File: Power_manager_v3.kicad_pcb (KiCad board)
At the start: 4 copper layers, 50 x 25 mm, 94 parts, among them J1 L_input, J2 Pow_mng_pow, J3 Load1, J4 Load2, J5 SWD (PLS5), J6 Dig_mod_iface, Q1 2N5551S, Q2 2N5551S, Q3 BSS138, U1 DC12003, U2 G3MB-202PL, U3 G3MB-202PL, U4 STM32F030F4Px, U5 HLW8112, U6 ADuM1251ARZ, U7 ADuM1201AR, U8 LM1117-3.3, Y1 CSTCE8M, Y2 ABLS-3.579545MHZ-D-3-Y-T

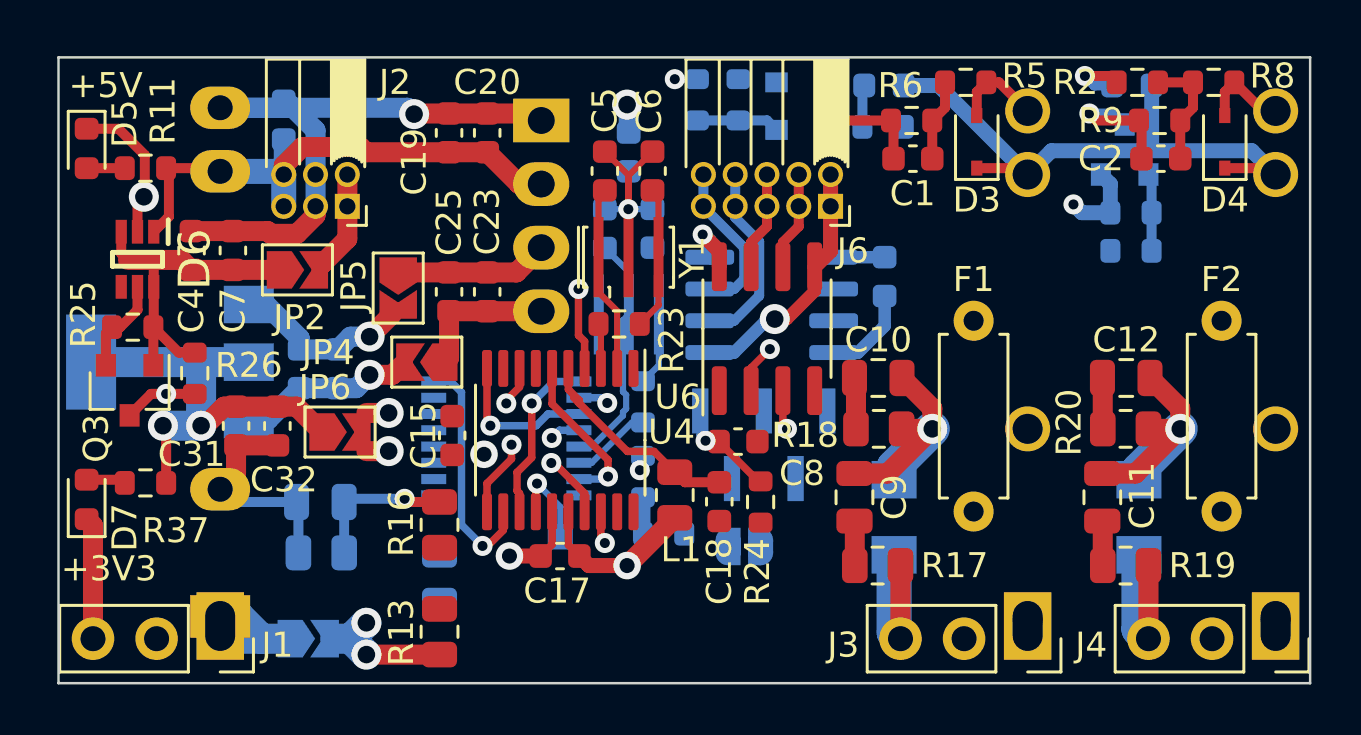
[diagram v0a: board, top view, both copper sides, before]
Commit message: Окончена трассировка печатной платы
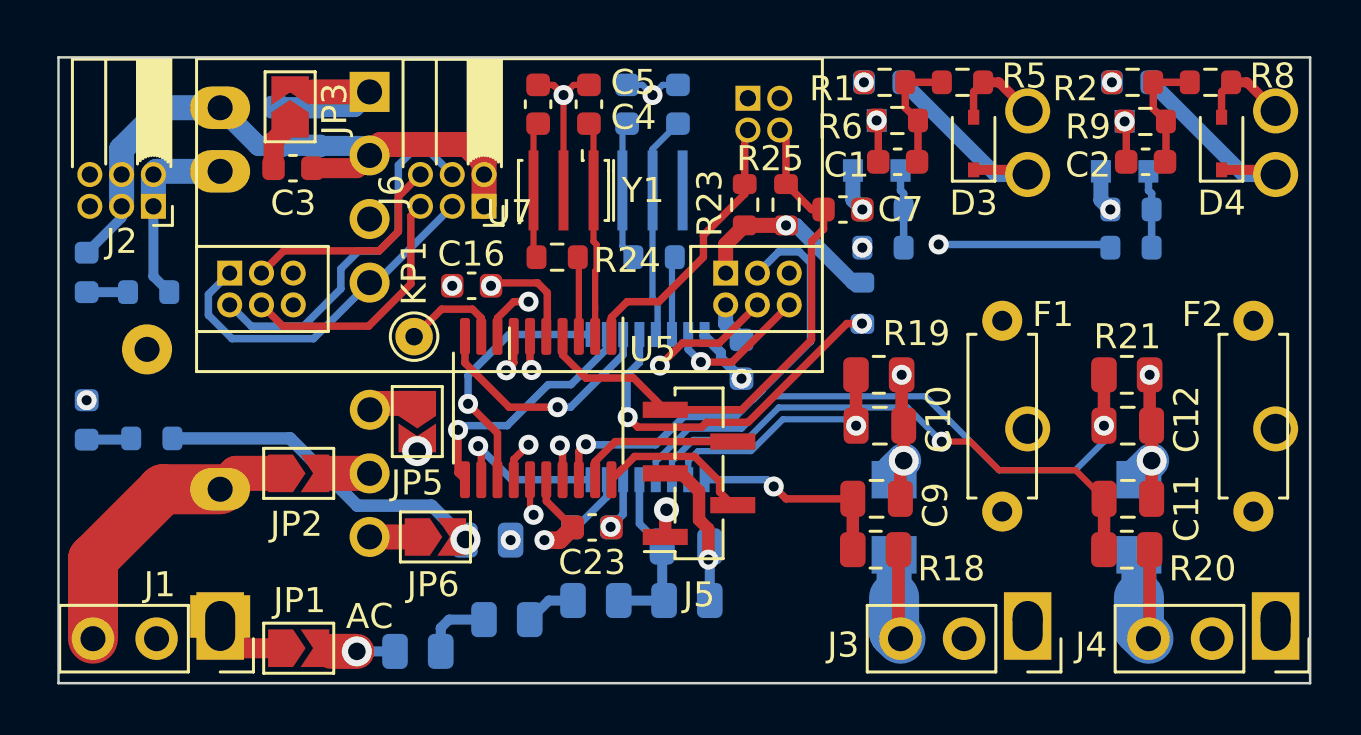
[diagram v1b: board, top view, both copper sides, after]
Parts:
- removed C19, C25, C27, C32: 10uF, Capacitor_SMD:C_0603_1608Metric
- removed C20, C24, C28, C30, C31: 100nF, Capacitor_SMD:C_0603_1608Metric
- removed C21, C22: 22pF, Capacitor_SMD:C_0603_1608Metric
- removed D7: +3.3V, LED_SMD:LED_0603_1608Metric
- removed PS1: B0505S, Modules:B0505S
- removed Q3: BSS138, Package_TO_SOT_SMD:SOT-23
- removed the R16 at (90.2, 93.7)
- removed the R21 at (85.5, 94.8)
- removed R28, R37: 10k, Resistor_SMD:R_0603_1608Metric
- removed U8: LM1117-3.3, Package_TO_SOT_SMD:SOT-223-3_TabPin2
- added C14: 100nF, Capacitor_SMD:C_0603_1608Metric, B.Cu at (96.3, 93.8)
- added C16: 100nF, Capacitor_SMD:C_0603_1608Metric, F.Cu at (91.5, 84.1)
- added GND1: TestPoint_Small, TestPoint:TestPoint_THTPad_D2.0mm_Drill1.0mm, B.Cu at (78.5, 86.7)
- added R14: 10k, Resistor_SMD:R_0603_1608Metric, B.Cu at (78.7, 90.2)
- added R17: 332k, Resistor_SMD:R_0805_2012Metric, B.Cu at (96.5, 96.7)
- C15, C8, L1: moved to B.Cu
- C17, C18: value 100nF -> 22pF; moved to B.Cu
- C3, J5, JP1, R1: moved to F.Cu
- C4: value 100nF -> 10pF
- C6: value 10pF -> 10uF; moved to B.Cu
- C7: value 10uF -> 100nF
- D5: value +5P -> +5V; moved to B.Cu
- D6: value LM66100DCKR -> +3.3VP; footprint Modules:SOP65P210X110-6N -> LED_SMD:LED_0603_1608Metric; moved to B.Cu
- J6: footprint Connector_PinSocket_1.27mm:PinSocket_2x05_P1.27mm_Horizontal -> Connector_PinSocket_1.27mm:PinSocket_2x03_P1.27mm_Horizontal
- JP2: value 5V_en -> N_en
- JP3: value BOOT0 -> 5V_en; footprint Jumper:SolderJumper-2_P1.3mm_Open_RoundedPad1.0x1.5mm -> Jumper:SolderJumper-2_P1.3mm_Open_TrianglePad1.0x1.5mm; moved to F.Cu
- JP4: value 5VL_en -> Jumper_2x2_Open; footprint Jumper:SolderJumper-2_P1.3mm_Open_TrianglePad1.0x1.5mm -> Modules:PinHeader_2x02_P1.27mm_Vertical; moved to B.Cu
- JP5: value N_en -> 5VP_en
- JP6: value 3V3_en -> 3.3VP_en
- KP1: footprint TestPoint:TestPoint_Pad_1.0x1.0mm -> TestPoint:TestPoint_THTPad_D1.5mm_Drill0.7mm; moved to F.Cu
- R11: value 10k -> 332k; footprint Resistor_SMD:R_0603_1608Metric -> Resistor_SMD:R_0805_2012Metric; moved to B.Cu
- R13: value 332k -> 10k; footprint Resistor_SMD:R_0805_2012Metric -> Resistor_SMD:R_0603_1608Metric; moved to B.Cu
- R22: value 10k -> 1k; footprint Resistor_SMD:R_0603_1608Metric -> Resistor_SMD:R_0805_2012Metric
- R23, R27: value 50 -> 10k
- R24: value 10k -> 50
- R26: value 2.2M -> 50; moved to B.Cu
- U4: value STM32F030F4Px -> DC5V_DC5V3V3_v3; footprint Package_SO:TSSOP-20_4.4x6.5mm_P0.65mm -> Modules:DC5V_DC5V3V3_v3; moved to B.Cu
- U5: value HLW8112 -> STM32F030F4Px; footprint Package_SO:SSOP-16_4.4x5.2mm_P0.65mm -> Package_SO:TSSOP-20_4.4x6.5mm_P0.65mm; moved to F.Cu
- U6: value ADuM1251ARZ -> HLW8112; footprint Package_SO:SOIC-8_3.9x4.9mm_P1.27mm -> Package_SO:SSOP-16_4.4x5.2mm_P0.65mm; moved to B.Cu
- U7: value ADuM1201AR -> ADuM_I2C_v3; footprint Package_SO:SOIC-8_3.9x4.9mm_P1.27mm -> Modules:ADuM_I2C_Horizontal; moved to F.Cu
- moved R25 26.6 mm to (104.1, 80.9), turned to 90 degrees
- moved JP3 25.3 mm to (84.3, 77.0), turned to 90 degrees
- moved C7 24.4 mm to (106.3, 81.1), turned to 0 degrees
- moved R11 23.1 mm to (92.9, 97.5), turned to 180 degrees
- moved C8 22.3 mm to (83.7, 77.8), turned to 90 degrees
- moved R26 18.9 mm to (98.8, 83.0), turned to 180 degrees
- moved C17 18.7 mm to (99.7, 76.9), turned to 270 degrees
- moved R13 17.9 mm to (78.6, 84.4), turned to 0 degrees
- moved C4 16.9 mm to (96.2, 76.9), turned to 90 degrees
- moved JP4 16.6 mm to (102.5, 76.6), turned to 270 degrees
- moved C18 16.3 mm to (97.7, 76.9), turned to 270 degrees
- moved C13 14.7 mm to (100.1, 94.5), turned to 180 degrees
- moved J6 13.8 mm to (92.0, 81.0)
- moved C6 13.6 mm to (85.3, 77.8)
- moved R24 12.7 mm to (94.9, 83.0), turned to 0 degrees
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- renumbered R14 to R15, R15 to R16, R17 to R18, R18 to R19, R19 to R20, R20 to R21
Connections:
- C15 pad 2: Net-(C15-Pad2) -> +3.3VP
- C17 pad 2: +3.3VP -> Net-(C17-Pad2)
- C23 pad 1: Net-(C23-Pad1) -> +3.3VP
- C23 pad 2: Net-(C23-Pad2) -> GNDPWR
- C3 pad 2: +5P -> +5V
- C4 pad 1: GND1 -> Net-(C4-Pad1)
- C4 pad 2: /+5P0 -> GNDPWR
- C6 pad 1: Net-(C6-Pad1) -> GND1
- C6 pad 2: GNDPWR -> Net-(C6-Pad2)
- C7 pad 1: GND1 -> /nRst
- C7 pad 2: /+5P0 -> GNDPWR
- C8 pad 1: /nRst -> GND1
- C8 pad 2: GNDPWR -> Net-(C6-Pad2)
- D1 pad 2: +5VL -> +5VP
- D2 pad 2: +5VL -> +5VP
- D3 pad 1: +5VL -> +5VP
- D4 pad 1: +5VL -> +5VP
- D6 pad 1: +5P -> GNDPWR
- D6 pad 2: GND1 -> Net-(D6-Pad2)
- J1 pad 2: Net-(J1-Pad2) -> (no net)
- J1 pad 3: GNDPWR -> Net-(J1-Pad3)
- J2 pad 1: +5VP -> +5V
- J2 pad 2: +5VP -> +5V
- J3 pad 2: Net-(J3-Pad2) -> (no net)
- J4 pad 2: Net-(J4-Pad2) -> (no net)
- J6 pad 3: /scl0 -> /+5V_state
- J6 pad 4: /scl0 -> /I2C_Int
- J6 pad 5: /sda0 -> /scl0
- JP2 pad 1: /+5P0 -> Net-(J1-Pad3)
- JP2 pad 2: +5VP -> GNDPWR
- JP3 pad 1: GNDPWR -> +5V
- JP3 pad 2: Net-(JP3-Pad2) -> Net-(C6-Pad2)
- JP4 pad 1: Net-(C23-Pad2) -> GNDPWR
- JP4 pad 2: +5VL -> Net-(JP4-Pad2)
- JP5 pad 1: Net-(C23-Pad1) -> Net-(JP5-Pad1)
- JP5 pad 2: GNDPWR -> +5VP
- JP6 pad 1: Net-(C31-Pad2) -> Net-(JP6-Pad1)
- L1 pad 2: Net-(C18-Pad2) -> Net-(C16-Pad2)
- R11 pad 1: Net-(D5-Pad2) -> Net-(R11-Pad1)
- R11 pad 2: +5P -> Net-(R11-Pad2)
- R12 pad 1: Net-(R12-Pad1) -> Net-(R11-Pad2)
- R12 pad 2: Net-(R12-Pad2) -> AC
- R13 pad 1: Net-(R12-Pad2) -> Net-(D5-Pad2)
- R13 pad 2: AC -> +5V
- R22 pad 1: Net-(JP3-Pad2) -> Net-(C13-Pad2)
- R22 pad 2: +3.3VP -> GNDPWR
- R23 pad 1: Net-(C6-Pad1) -> Net-(JP4-Pad2)
- R23 pad 2: Net-(R23-Pad2) -> +3.3VP
- R24 pad 1: +3.3VP -> Net-(C5-Pad1)
- R24 pad 2: /nRst -> Net-(R24-Pad2)
- R25 pad 1: /+5P0 -> +3.3VP
- R25 pad 2: Net-(D6-Pad5) -> /nRst
- R26 pad 1: /+5V_state -> Net-(R26-Pad1)
- R26 pad 2: /+5P0 -> Net-(C18-Pad2)
- R27 pad 1: Net-(R27-Pad1) -> +3.3VP
- R27 pad 2: Net-(C22-Pad2) -> Net-(R27-Pad2)
- U1 pad 2: GNDPWR -> Net-(J1-Pad3)
- U1 pad 3: +5P -> +5V
- U2 pad 3: +5VL -> +5VP
- U3 pad 3: +5VL -> +5VP
- U4 pad 1: Net-(JP3-Pad2) -> Net-(C6-Pad2)
- U4 pad 2: Net-(C5-Pad1) -> GND1
- U4 pad 3: Net-(R23-Pad2) -> +5P
- U4 pad 4: /nRst -> /+5V_state
- U4 pad 5: Net-(C18-Pad2) -> Net-(JP5-Pad1)
- U4 pad 6: /Int -> GNDPWR
- U4 pad 7: /+5V_valid -> Net-(JP6-Pad1)
- U5 pad 1: Net-(C9-Pad2) -> Net-(JP4-Pad2)
- U5 pad 10: /SPI_SCLK -> /SPI_SSEL
- U5 pad 11: /SPI_SSEL -> /SPI_SCLK
- U5 pad 12: Net-(R28-Pad2) -> /SPI_MISO
- U5 pad 13: Net-(C21-Pad2) -> /SPI_MOSI
- U5 pad 14: Net-(R27-Pad1) -> /+5V_valid
- U5 pad 15: /Int -> GNDPWR
- U5 pad 2: Net-(C10-Pad1) -> Net-(C4-Pad1)
- U5 pad 3: Net-(C11-Pad2) -> Net-(R24-Pad2)
- U5 pad 4: Net-(C12-Pad1) -> /nRst
- U5 pad 5: Net-(C13-Pad2) -> Net-(C16-Pad2)
- U5 pad 6: GNDPWR -> /Int
- U5 pad 7: Net-(C15-Pad2) -> /L1_o1_nEn
- U5 pad 8: /SPI_MISO -> /L1_o2_nEn
- U5 pad 9: /SPI_MOSI -> Net-(KP1-Pad1)
- U6 pad 1: +3.3VP -> Net-(C9-Pad2)
- U6 pad 2: /I2C_SDA -> Net-(C10-Pad1)
- U6 pad 3: /I2C_SCL -> Net-(C11-Pad2)
- U6 pad 4: GNDPWR -> Net-(C12-Pad1)
- U6 pad 5: GND1 -> Net-(C13-Pad2)
- U6 pad 6: /scl0 -> GNDPWR
- U6 pad 7: /sda0 -> Net-(C14-Pad2)
- U6 pad 8: +5VP -> /SPI_MISO
- Y1 pad 1: Net-(C5-Pad1) -> Net-(C4-Pad1)
- Y1 pad 3: Net-(C6-Pad1) -> Net-(C5-Pad1)
- Y2 pad 1: Net-(C22-Pad2) -> Net-(C18-Pad2)
- Y2 pad 2: Net-(C21-Pad2) -> Net-(C17-Pad2)
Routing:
- net GNDPWR: track 61.2 -> 147.9 mm, vias 7 -> 13
- net AC: track 83.2 -> 41.7 mm, vias 2 -> 1
- net +5VP: track 20.8 -> 58.6 mm, vias 2 -> 1
- net +3.3VP: track 15.3 -> 51.5 mm, vias 3 -> 5
- net +5VL: track 31.3 -> 0.00 mm, vias 1 -> 0
- net /L1_o2_nEn: track 0.00 -> 27.0 mm, vias 0 -> 2
- net Net-(C12-Pad1): track 2.04 -> 24.1 mm, vias 0 -> 1
- net Net-(C11-Pad2): track 1.79 -> 22.4 mm, vias 0 -> 1
- net Net-(C31-Pad2): track 18.3 -> 0.00 mm, vias 2 -> 0
- net /+5V_valid: track 0.00 -> 17.7 mm, vias 0 -> 1
- net Net-(C16-Pad2): track 0.00 -> 15.2 mm, vias 0 -> 2
- net Net-(R27-Pad2): track 0.00 -> 14.8 mm, vias 0 -> 2
- net /+5P0: track 14.6 -> 0.00 mm
- net Net-(J1-Pad3): track 0.00 -> 12.1 mm
- net Net-(JP4-Pad2): track 0.00 -> 11.2 mm
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- removed copper zone on In2.Cu, net GNDPWR
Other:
- net class AC230V removed
- net class Digital added: clearance 0.2, trace_width 0.3, via_dia 0.8, via_drill 0.4
- board text added: "+3.3V"
- board text removed: "+3V3"
